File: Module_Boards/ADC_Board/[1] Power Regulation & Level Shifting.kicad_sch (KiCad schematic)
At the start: 26 parts, among them U2 TXB0104RUTR, U3 TPS22916CYFPR, U4 TPS7A9401DSCR

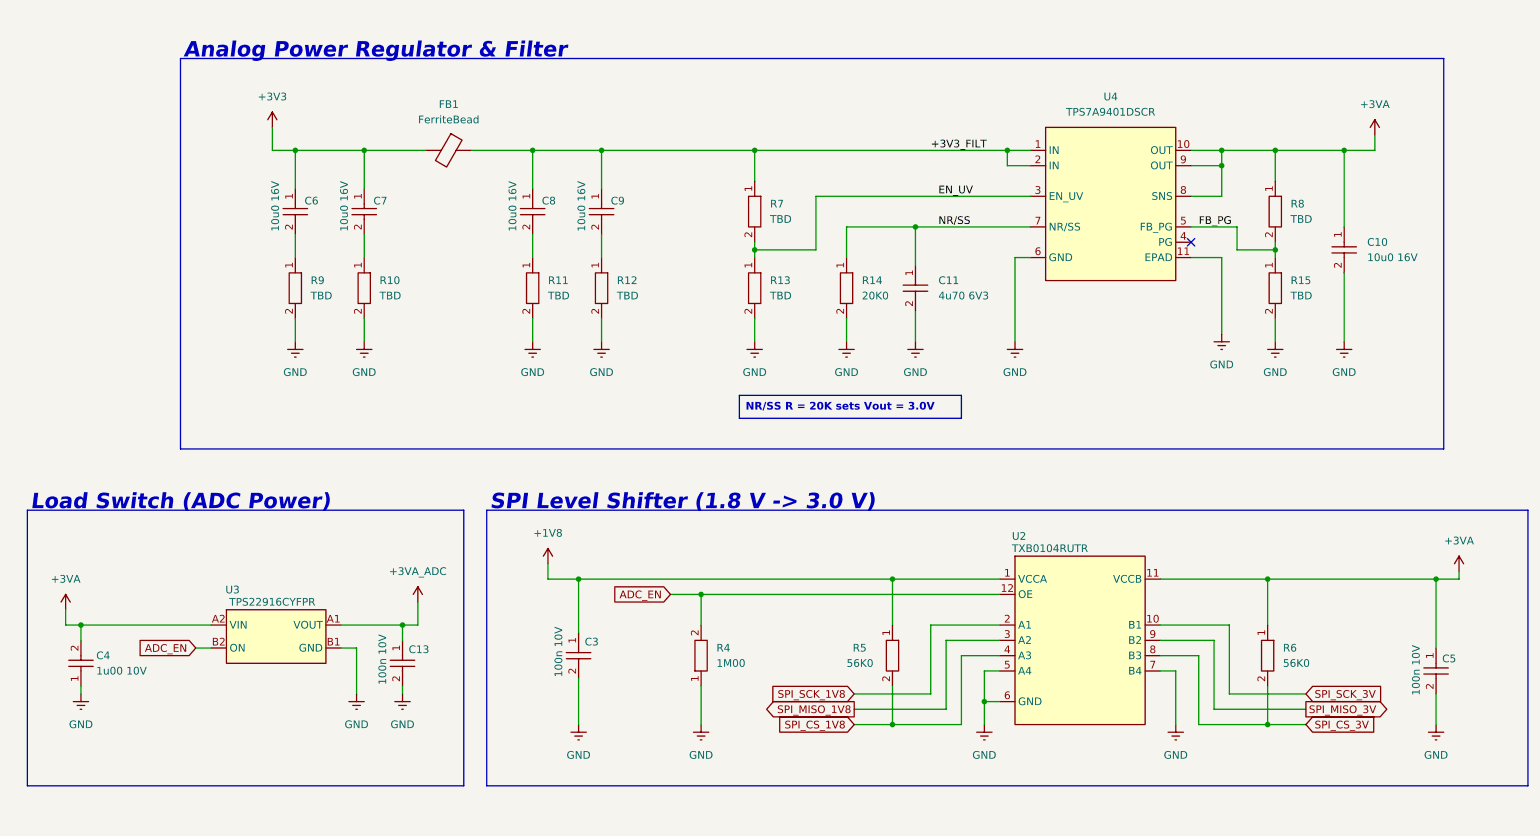
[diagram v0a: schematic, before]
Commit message: Big push. Fixed the issues that were pending. See github
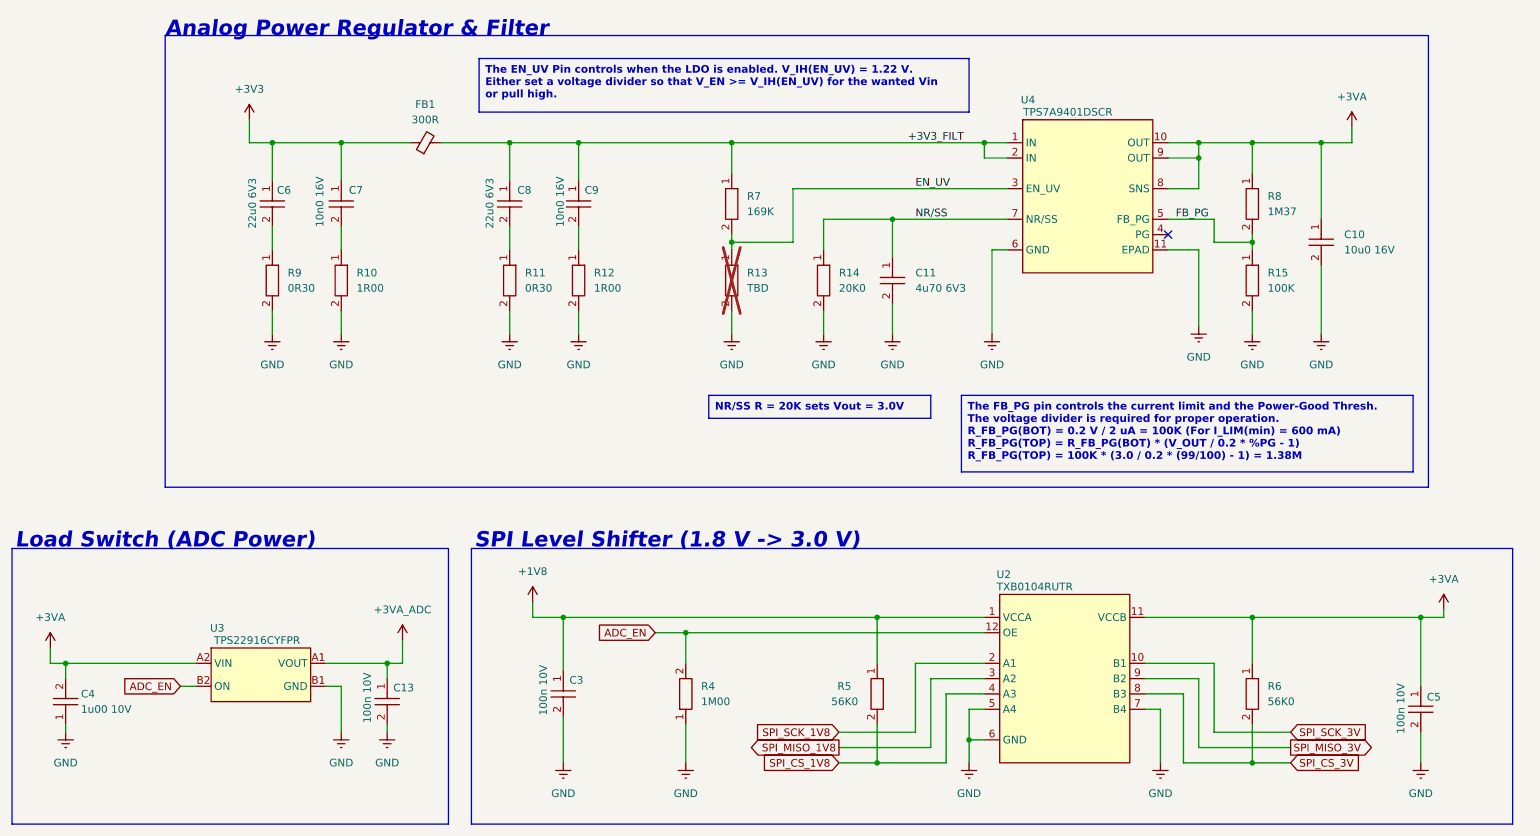
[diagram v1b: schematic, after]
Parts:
- removed C6, C9: 10u0 16V, X-MODs_PcbLib:C0402, symbol X-MODs_SchLib:GRM155R60G106ME01D
- added C6: 22u0 6V3, X-MODs_PcbLib:C0402, symbol X-MODs_SchLib:CL05A226MQ5CUN
- added C9: 10n0 16V, X-MODs_PcbLib:C0402, symbol X-MODs_SchLib:CL05B103JO5NNWC
- C7: value 10u0 16V -> 10n0 16V; symbol X-MODs_SchLib:GRM155R60G106ME01D -> X-MODs_SchLib:CL05B103JO5NNWC; MPN GRM155R60G106ME01D -> CL05B103JO5NNWC
- C8: value 10u0 16V -> 22u0 6V3; symbol X-MODs_SchLib:GRM155R60G106ME01D -> X-MODs_SchLib:CL05A226MQ5CUN; MPN GRM155R60G106ME01D -> CL05A226MQ5CUN
- FB1: value FerriteBead -> 300R; symbol Device:FerriteBead -> X-MODs_SchLib:LI0402B301R-10; MPN (none) -> LI0402B301R-10
- R10, R12: value TBD -> 1R00; symbol X-MODs_SchLib:R -> X-MODs_SchLib:CRCW04021R00FKEDHP; MPN (none) -> CRCW04021R00FKEDHP
- R11, R9: value TBD -> 0R30; symbol X-MODs_SchLib:R -> X-MODs_SchLib:ERJ-2BQJR30X; MPN (none) -> ERJ-2BQJR30X
- R13: now not fitted
- R15: value TBD -> 100K; symbol X-MODs_SchLib:R -> X-MODs_SchLib:CRCW0402100KFKEDC; MPN (none) -> CRCW0402100KFKEDC
- R7: value TBD -> 169K; symbol X-MODs_SchLib:R -> X-MODs_SchLib:CRCW0402169KFKTD; MPN (none) -> CRCW0402169KFKTD
- R8: value TBD -> 1M37; symbol X-MODs_SchLib:R -> X-MODs_SchLib:CRCW04021M37FKED; MPN (none) -> CRCW04021M37FKED
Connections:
- net +3V3: now also FB1.1, C6.1; no longer FB1.2
- net +3V3_FILT: now also FB1.2, C9.1; no longer FB1.1
- net at R12.1: now also C9.2
- net at R9.1: now also C6.2
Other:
- moved on the sheet: C10, C11, C13, C3, C4, C5, C7, C8, FB1, R10, R11, R12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
